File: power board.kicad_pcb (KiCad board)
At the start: 2 copper layers, 226.1 x 95.9 mm, 30 parts, among them J1 Conn_01x02_Female, J10 Conn_01x02_Female, J11 Conn_01x02_Female, J12 Conn_01x02_Female, J2 Conn_01x02_Female, J3 Conn_01x02_Female, J4 Conn_01x02_Female, J5 Conn_01x02_Female, J6 Conn_01x02_Female, J7 Conn_01x02_Female, J8 Conn_01x02_Female, J9 Conn_01x02_Female, Q1 STP160N3LL, U1 THL-25-2411

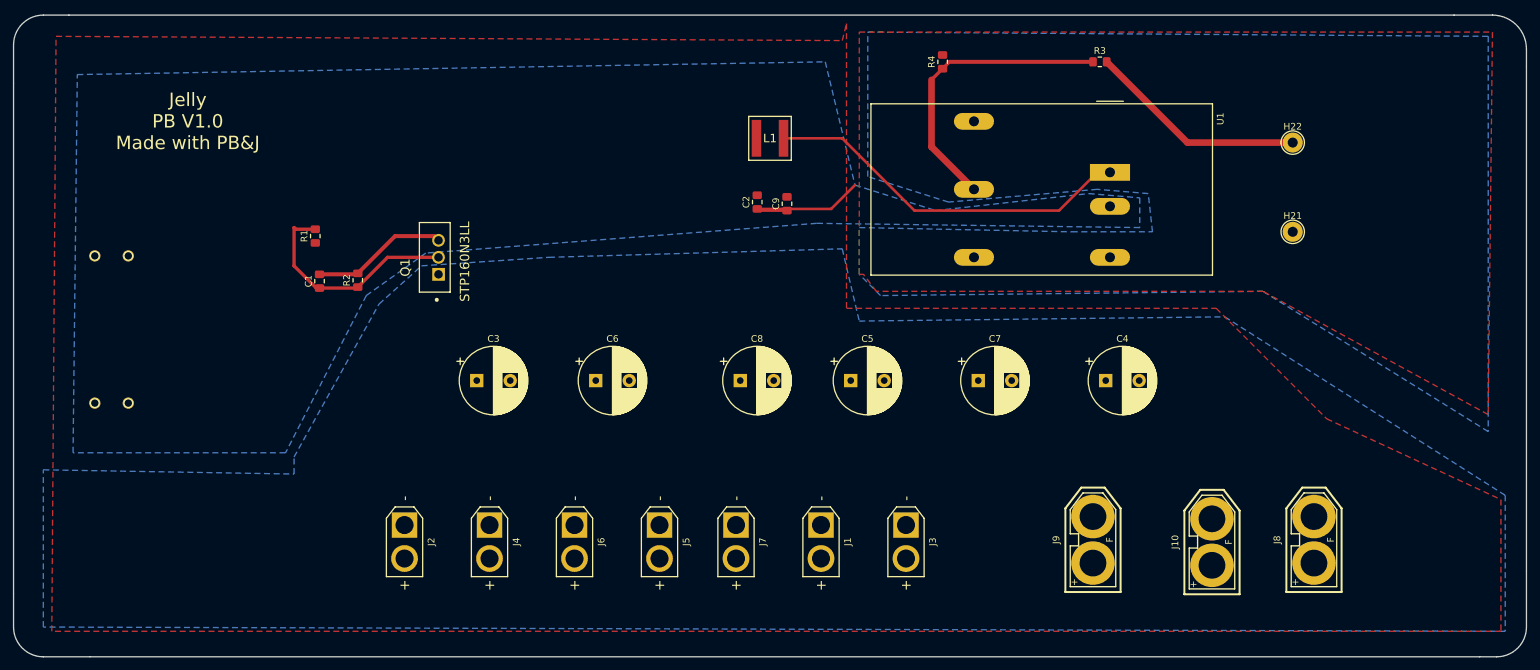
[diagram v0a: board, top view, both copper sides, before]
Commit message: final V1.0 sent out -gerbers zipped
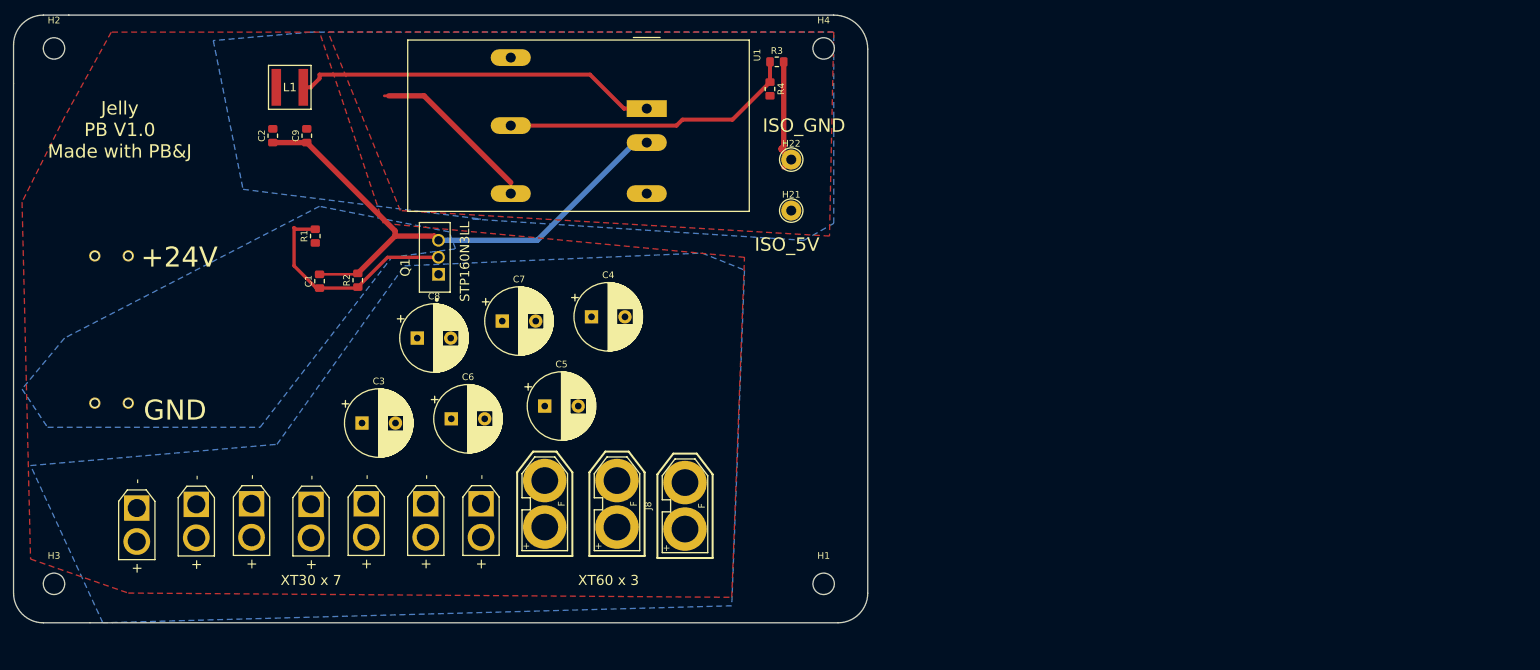
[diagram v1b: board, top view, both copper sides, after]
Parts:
- added H1: MountingHole, MountingHole:MountingHole_3.2mm_M3, F.Cu at (142.0, 118.0)
- added H2: MountingHole, MountingHole:MountingHole_3.2mm_M3, F.Cu at (27.0, 38.0)
- added H3: MountingHole, MountingHole:MountingHole_3.2mm_M3, F.Cu at (27.0, 118.0)
- added H4: MountingHole, MountingHole:MountingHole_3.2mm_M3, F.Cu at (142.0, 38.0)
- moved J8 94.1 mm to (121.3, 106.3)
- moved J10 89.1 mm to (111.1, 106.0)
- moved J9 82.1 mm to (100.3, 106.0)
- moved C4 77.4 mm to (107.3, 78.1)
- moved H21 75.0 mm to (137.2, 62.2)
- moved H22 75.0 mm to (137.2, 54.6)
- moved C2 73.1 mm to (59.7, 51.0)
- moved C9 72.5 mm to (64.8, 51.0)
- moved L1 72.2 mm to (62.2, 43.8)
- moved C7 71.7 mm to (94.0, 78.7)
- moved U1 69.9 mm to (115.6, 47.0)
- moved J3 63.6 mm to (90.8, 106.0)
- moved J1 59.1 mm to (82.5, 106.0)
- moved J7 55.3 mm to (73.7, 106.0)
- moved J5 52.2 mm to (65.4, 106.1)
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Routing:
- net GND: track 41.0 -> 82.3 mm
- net ISO_GND_5V: track 32.8 -> 43.2 mm
- net Net-(R3-Pad1): track 44.2 -> 45.4 mm
- net Net-(L1-Pad2): track 55.6 -> 54.6 mm
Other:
- board size 226.1 x 95.9 mm -> 127.6 x 90.8 mm
- board text added: "+24V"
- board text added: "GND"
- board text added: "ISO_5V"
- board text added: "ISO_GND"
- board text added: "XT30 x 7"
- board text added: "XT60 x 3"
